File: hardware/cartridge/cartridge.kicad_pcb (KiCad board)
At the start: 2 copper layers, 93.9 x 85.1 mm, 14 parts, among them J1 MX29LV320EBTI-70G, J2 FM28V100-TG, J3 SN74LVC8T245PWR, J4 MX29 pins 1-24, J5 MX29 pins 25-48, J6 FRAM pins 1-16, J7 FRAM pins 17-32, J8 Conn_01x12, J9 Conn_01x12

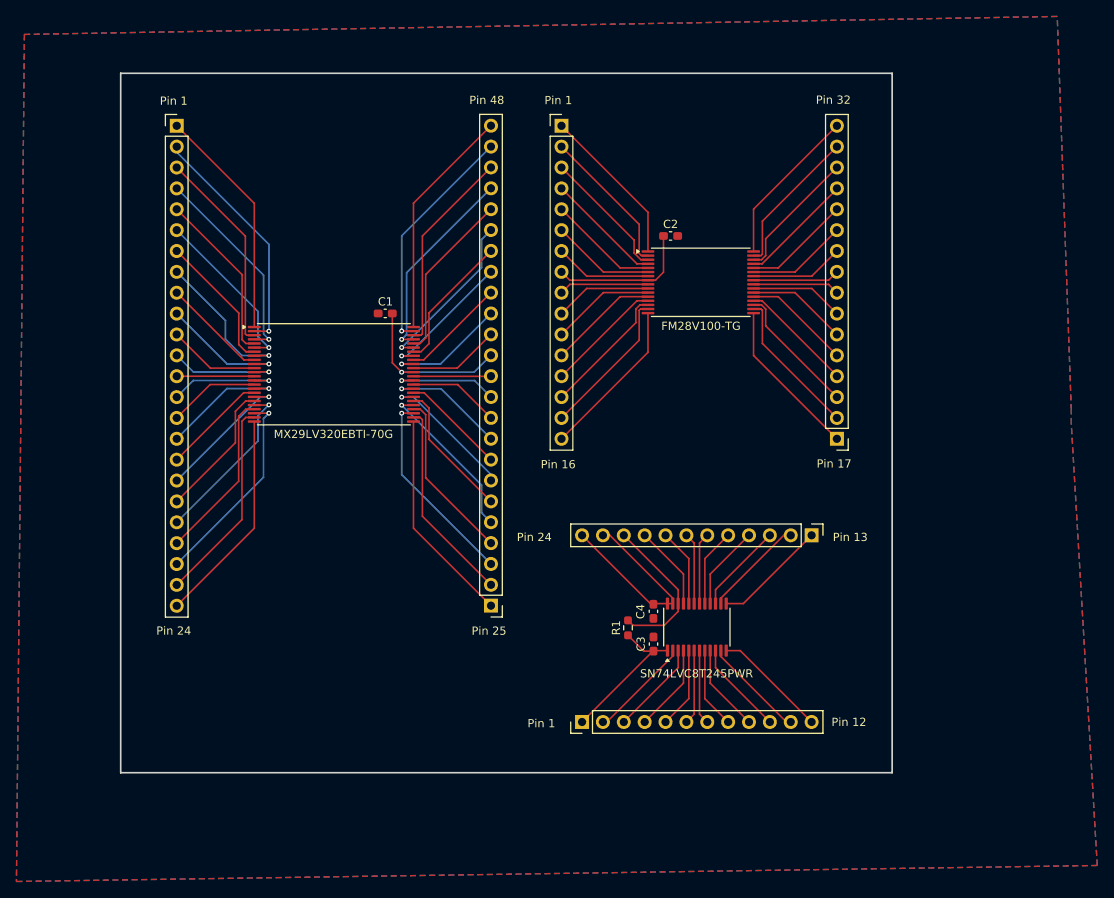
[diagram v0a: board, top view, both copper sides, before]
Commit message: Add PCB
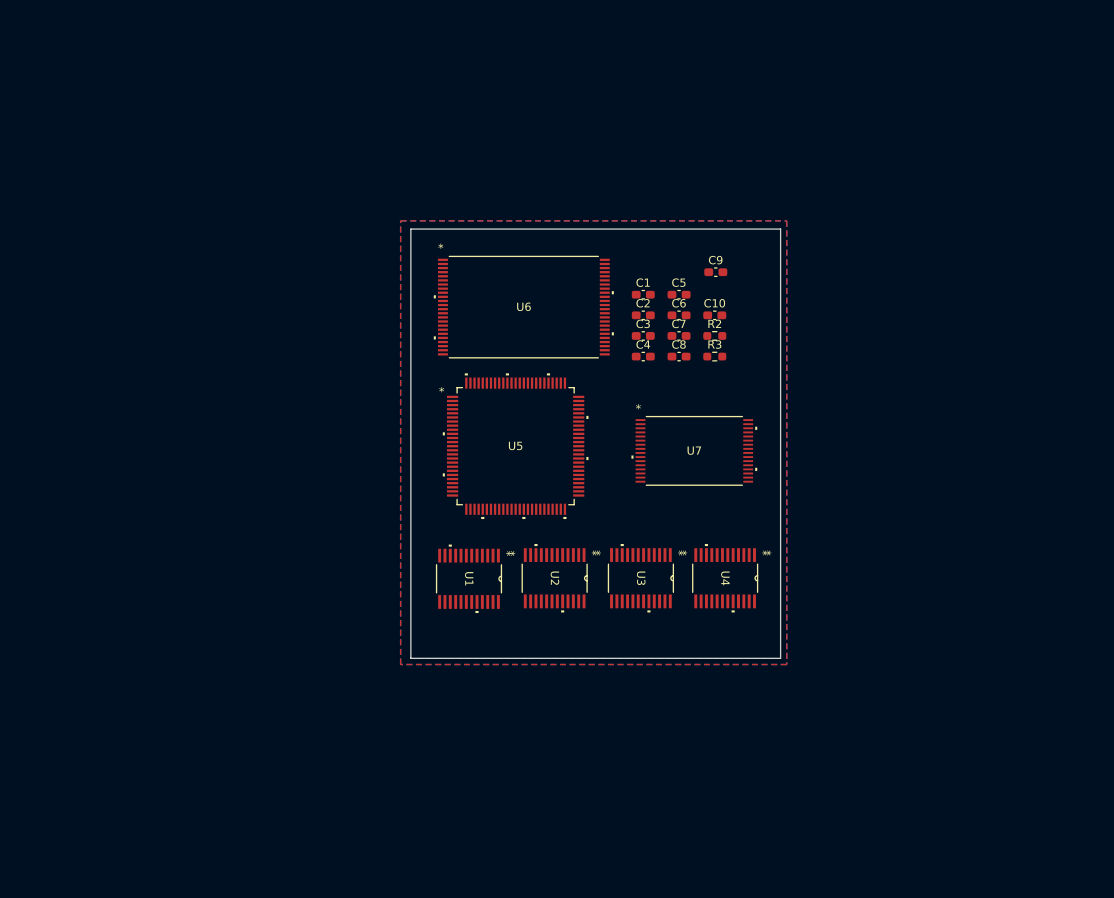
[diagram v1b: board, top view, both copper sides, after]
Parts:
- removed J1: MX29LV320EBTI-70G, Package_SO:TSOP-I-48_18.4x12mm_P0.5mm
- removed J2: FM28V100-TG, Package_SO:TSOP-I-32_11.8x8mm_P0.5mm
- removed J3: SN74LVC8T245PWR, Package_SO:TSSOP-24_4.4x7.8mm_P0.65mm
- removed J4: MX29 pins 1-24, Connector_PinHeader_2.54mm:PinHeader_1x24_P2.54mm_Vertical
- removed J5: MX29 pins 25-48, Connector_PinHeader_2.54mm:PinHeader_1x24_P2.54mm_Vertical
- removed J6: FRAM pins 1-16, Connector_PinHeader_2.54mm:PinHeader_1x16_P2.54mm_Vertical
- removed J7: FRAM pins 17-32, Connector_PinHeader_2.54mm:PinHeader_1x16_P2.54mm_Vertical
- removed J8, J9: Conn_01x12, Connector_PinHeader_2.54mm:PinHeader_1x12_P2.54mm_Vertical
- removed R1: 10K, Resistor_SMD:R_0603_1608Metric_Pad0.98x0.95mm_HandSolder
- added C10: 100nF, Capacitor_SMD:C_0603_1608Metric_Pad1.08x0.95mm_HandSolder, F.Cu at (165.5, 54.8)
- added C5: 100nF, Capacitor_SMD:C_0603_1608Metric_Pad1.08x0.95mm_HandSolder, F.Cu at (161.1, 52.2)
- added C6: 100nF, Capacitor_SMD:C_0603_1608Metric_Pad1.08x0.95mm_HandSolder, F.Cu at (161.1, 54.8)
- added C7: 100nF, Capacitor_SMD:C_0603_1608Metric_Pad1.08x0.95mm_HandSolder, F.Cu at (161.1, 57.3)
- added C8: 100nF, Capacitor_SMD:C_0603_1608Metric_Pad1.08x0.95mm_HandSolder, F.Cu at (161.1, 59.8)
- added C9: 100nF, Capacitor_SMD:C_0603_1608Metric_Pad1.08x0.95mm_HandSolder, F.Cu at (165.6, 49.5)
- added R2: 10K, Resistor_SMD:R_0603_1608Metric_Pad0.98x0.95mm_HandSolder, F.Cu at (165.5, 57.3)
- added R3: 10K, Resistor_SMD:R_0603_1608Metric_Pad0.98x0.95mm_HandSolder, F.Cu at (165.5, 59.8)
- added U1: SN74LVC8T245PWR, SN74LVC8T245PWR:PW24, F.Cu at (135.6, 86.8)
- added U2: SN74LVC8T245PWR, SN74LVC8T245PWR:PW24, F.Cu at (146.0, 86.8)
- added U3: SN74LVC8T245PWR, SN74LVC8T245PWR:PW24, F.Cu at (156.5, 86.8)
- added U4: SN74LVC8T245PWR, SN74LVC8T245PWR:PW24, F.Cu at (166.8, 86.8)
- added U5: LCMXO2-1200HC-4TG100C, LCMXO2-1200HC-4TG100C:TQFP100_LAT, F.Cu at (141.3, 70.7)
- added U6: MX29LV320EBTI-70G, MX29LV320EBTI-70G:TSOPI48L12X20NORMAL_MAC, F.Cu at (142.3, 53.8)
- added U7: FM28V100-TG, FM28V100-TG:TSOP-32, F.Cu at (163.0, 71.2)
- moved C3 37.5 mm to (156.8, 57.3), turned to 0 degrees
- moved C1 31.5 mm to (156.8, 52.2), turned to 0 degrees
- moved C4 31.0 mm to (156.8, 59.8), turned to 0 degrees
- moved C2 10.2 mm to (156.8, 54.8)
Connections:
- C1 pad 1: Net-(J1-Pin_37) -> +3.3V
- C2 pad 1: Net-(J2-Pin_8) -> VCCB
- C3 pad 1: Net-(J3-Pin_1) -> +3.3V
- C4 pad 1: Net-(J3-Pin_23) -> VCCB
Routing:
- net GND: track 100.1 -> 0.00 mm, vias 1 -> 0
- net Net-(J1-Pin_2): track 28.9 -> 0.00 mm, vias 1 -> 0
- net Net-(J1-Pin_48): track 28.4 -> 0.00 mm
- net Net-(J1-Pin_1): track 28.4 -> 0.00 mm
- net Net-(J1-Pin_47): track 28.4 -> 0.00 mm, vias 1 -> 0
- net Net-(J3-Pin_23): track 26.8 -> 0.00 mm
- net Net-(J1-Pin_24): track 26.3 -> 0.00 mm
- net Net-(J1-Pin_25): track 26.3 -> 0.00 mm
- net Net-(J1-Pin_23): track 25.0 -> 0.00 mm
- net Net-(J1-Pin_3): track 24.9 -> 0.00 mm
- net Net-(J1-Pin_4): track 24.8 -> 0.00 mm, vias 1 -> 0
- net Net-(J1-Pin_22): track 24.8 -> 0.00 mm, vias 1 -> 0
- net Net-(J1-Pin_26): track 24.8 -> 0.00 mm
- net Net-(J1-Pin_45): track 24.3 -> 0.00 mm, vias 1 -> 0
- net Net-(J1-Pin_21): track 20.9 -> 0.00 mm
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- added copper zone on B.Cu, net (none)
- added copper zone on F.Cu, net (none)
- removed copper zone on B.Cu, net GND
- removed copper zone on F.Cu, net GND
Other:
- board size 93.9 x 85.1 mm -> 45 x 52.2 mm
- board text removed: "Pin 1"
- board text removed: "Pin 12"
- board text removed: "Pin 13"
- board text removed: "Pin 16"
- board text removed: "Pin 17"
- board text removed: "Pin 24"
- board text removed: "Pin 25"
- board text removed: "Pin 32"
- board text removed: "Pin 48"
